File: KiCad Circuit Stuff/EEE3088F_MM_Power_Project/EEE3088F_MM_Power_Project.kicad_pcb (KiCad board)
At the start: 2 copper layers, 79 parts, among them J1 Conn_01x02, J2 Conn_02x16_Odd_Even, U1 MT3608, U10 DRV8833PWP, U11 SS-12D06-G050, U12 AP22814AW5-7, U14 AP22814AW5-7, U2 INA219AIDCNR, U3 AMS1117-3.3, U4 TPS5430DDAR, U5 TP4056, U6 TS5A3159DCKR, U7 TYPE-C_16P_QTGM027, U8 DRV8833PWP, U9 HUSB237-AA001-DN06R

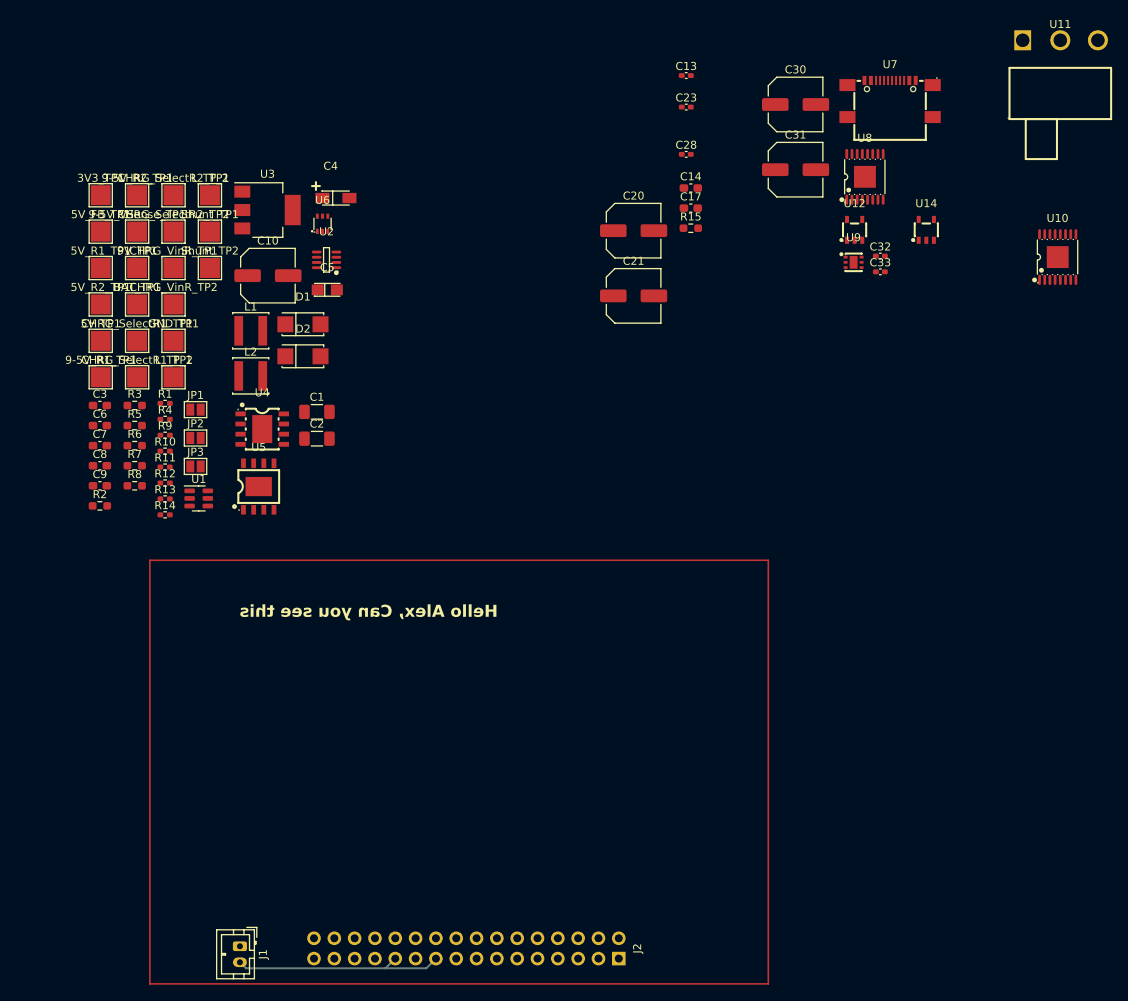
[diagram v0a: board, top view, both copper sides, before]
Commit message: Done Significant circuit work
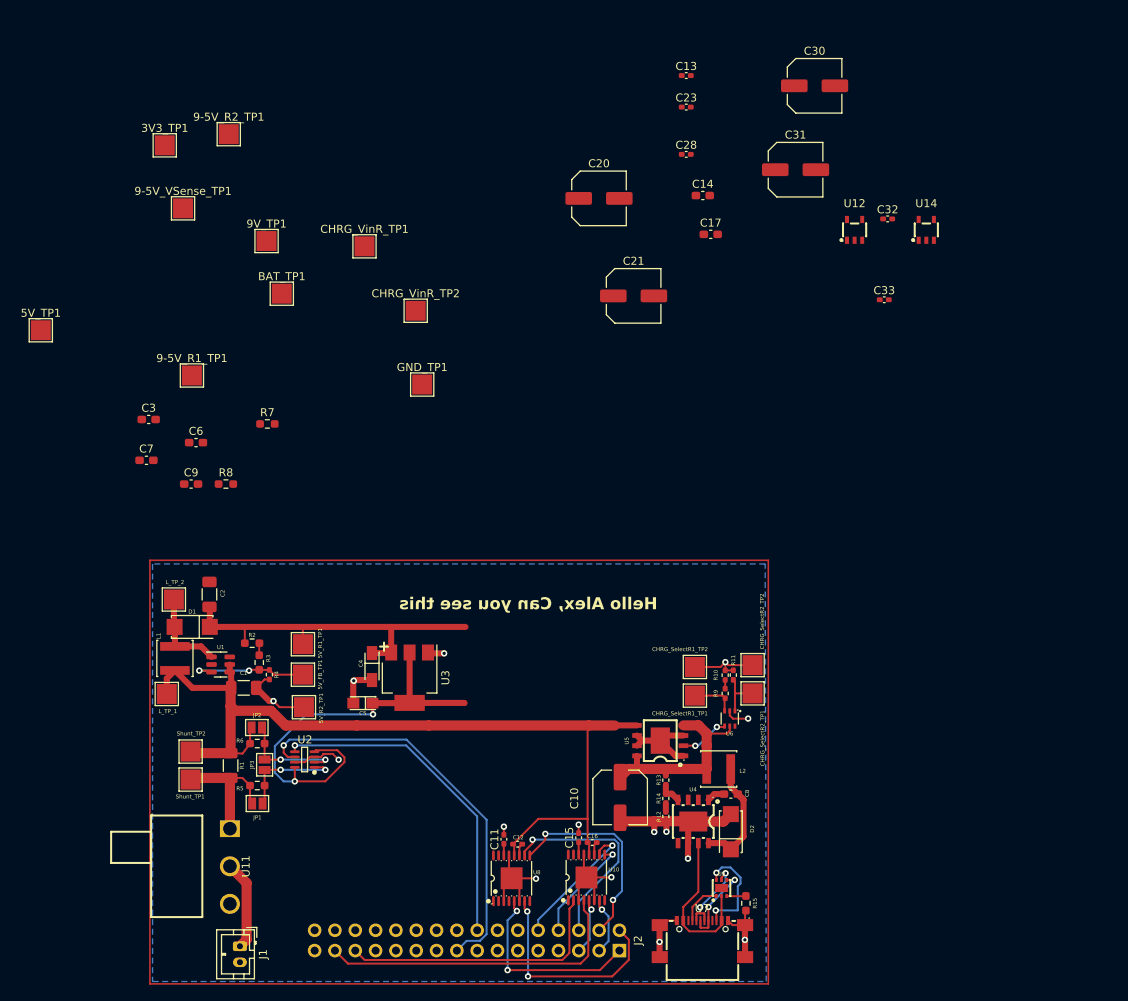
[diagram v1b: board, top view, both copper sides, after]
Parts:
- added C11: 2.2uF, Capacitor_SMD:C_0402_1005Metric_Pad0.74x0.62mm_HandSolder, F.Cu at (144.2, 134.9)
- added C12: 10nF, Capacitor_SMD:C_0402_1005Metric_Pad0.74x0.62mm_HandSolder, F.Cu at (146.0, 135.5)
- added C15: 2.2uF, Capacitor_SMD:C_0402_1005Metric_Pad0.74x0.62mm_HandSolder, F.Cu at (153.6, 134.7)
- added C16: 10nF, Capacitor_SMD:C_0402_1005Metric_Pad0.74x0.62mm_HandSolder, F.Cu at (155.3, 135.3)
- R1: footprint Resistor_SMD:R_0402_1005Metric_Pad0.72x0.64mm_HandSolder -> Resistor_SMD:R_1206_3216Metric_Pad1.30x1.75mm_HandSolder
- moved U11 146.4 mm to (110.0, 138.2), turned to -90 degrees
- moved U7 107.6 mm to (169.1, 147.3)
- moved U8 98.2 mm to (145.2, 139.8)
- moved U10 97.4 mm to (154.6, 139.6)
- moved CHRG_SelectR2_TP1 95.5 mm to (175.3, 116.6)
- moved CHRG_SelectR2_TP2 90.4 mm to (175.3, 113.1)
- moved C8 88.9 mm to (172.6, 129.2)
- moved R15 84.7 mm to (174.5, 142.9), turned to -90 degrees
- moved CHRG_SelectR1_TP1 82.6 mm to (168.1, 116.9)
- moved U6 80.1 mm to (172.5, 119.8), turned to 180 degrees
- moved D2 80.0 mm to (172.6, 133.9), turned to 90 degrees
- moved U9 79.9 mm to (171.4, 141.0), turned to 90 degrees
- moved C10 78.7 mm to (158.8, 129.6), turned to -90 degrees
- moved CHRG_SelectR1_TP2 78.6 mm to (168.1, 113.3)
- moved R9 77.1 mm to (171.9, 116.6), turned to 90 degrees
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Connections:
- C1 pad 1: /Battery_Out_After_Switch -> /Battery_Out
- C14 pad 1: /Battery_Out_After_Switch -> /Battery_Out
- C17 pad 1: /Battery_Out_After_Switch -> /Battery_Out
- C9 pad 2: /Battery_Out_Before_Switch -> /Battery_Out
- J1 pad 1: /Battery_In -> /Battery_In_Before_Switch
- J2 pad 14: /Battery_In -> /Battery_Out
- JP1 pad 1: /Battery_In -> /Battery_In_After_Switch
- JP2 pad 2: /Battery_Out_Before_Switch -> /Battery_Out
- L1 pad 1: /Battery_Out_After_Switch -> /Battery_Out
- L_TP_1 pad 1: /Battery_Out_After_Switch -> /Battery_Out
- R1 pad 1: /Battery_Out_Before_Switch -> /Battery_Out
- R1 pad 2: /Battery_In -> /Battery_In_After_Switch
- R5 pad 1: /Battery_In -> /Battery_In_After_Switch
- R6 pad 1: /Battery_Out_Before_Switch -> /Battery_Out
- Shunt_TP1 pad 1: /Battery_In -> /Battery_In_After_Switch
- Shunt_TP2 pad 1: /Battery_Out_Before_Switch -> /Battery_Out
- U1 pad 4: /Battery_Out_After_Switch -> /Battery_Out
- U1 pad 5: /Battery_Out_After_Switch -> /Battery_Out
- U10 pad 12: /Battery_Out_After_Switch -> /Battery_Out
- U10 pad 16: /AIN2 (U2) -> /AIN1 (U2)
- U11 pad 1: /Battery_Out_After_Switch -> /Battery_In_After_Switch
- U11 pad 2: /Battery_Out_Before_Switch -> /Battery_In_Before_Switch
- U5 pad 5: /Battery_Out_Before_Switch -> /Battery_Out
- U6 pad 5: +5V -> /Battey_Charger_VDD
- U7 pad A6: /DP2 -> /DP1
- U7 pad A7: /DN2 -> /DN1
- U8 pad 12: /Battery_Out_After_Switch -> /Battery_Out
- U9 pad 4: /DP1/DP2 -> /DP1
- U9 pad 5: /DN1/DN2 -> /DN1
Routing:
- net /Battery_Out: track 0.00 -> 113.1 mm
- net GND: track 27.0 -> 110.1 mm, vias 0 -> 15
- net +3V3: track 0.00 -> 53.2 mm, vias 0 -> 2
- net /I2C1_SDA: track 0.00 -> 51.2 mm, vias 0 -> 1
- net +5V: track 0.00 -> 44.4 mm
- net /I2C1_SCL: track 0.00 -> 41.5 mm, vias 0 -> 1
- net /AOUT2 (U2): track 0.00 -> 39.9 mm
- net /AOUT1 (U2): track 0.00 -> 34.4 mm
- net /BOUT1 (U1): track 0.00 -> 27.2 mm, vias 0 -> 2
- net /BIN2 (U1): track 0.00 -> 26.2 mm, vias 0 -> 1
- net /BIN1 (U1): track 0.00 -> 25.7 mm, vias 0 -> 2
- net /Battey_Charger_VDD: track 0.00 -> 25.2 mm
- net /BOUT2 (U1): track 0.00 -> 24.3 mm, vias 0 -> 2
- net +9V: track 0.00 -> 20.1 mm
- net /BIN2 (U2): track 0.00 -> 16.8 mm, vias 0 -> 1
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- added copper zone on B.Cu, net GND
